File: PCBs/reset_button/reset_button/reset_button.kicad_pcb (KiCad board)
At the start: 2 copper layers, 20 x 40 mm, 3 parts, among them J1 Conn_01x05, SW1 SW_DIP_x02, SW2 SW_DIP_x02

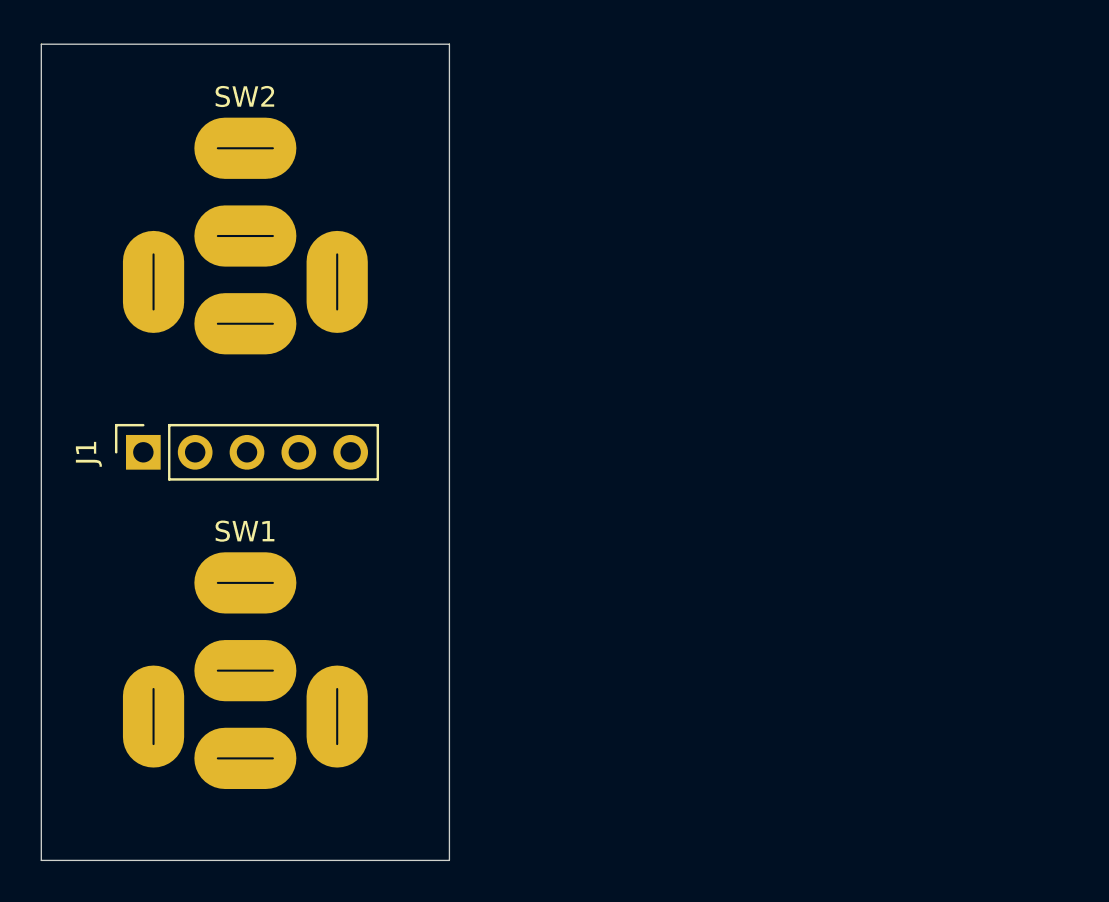
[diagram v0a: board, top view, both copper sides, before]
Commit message: update
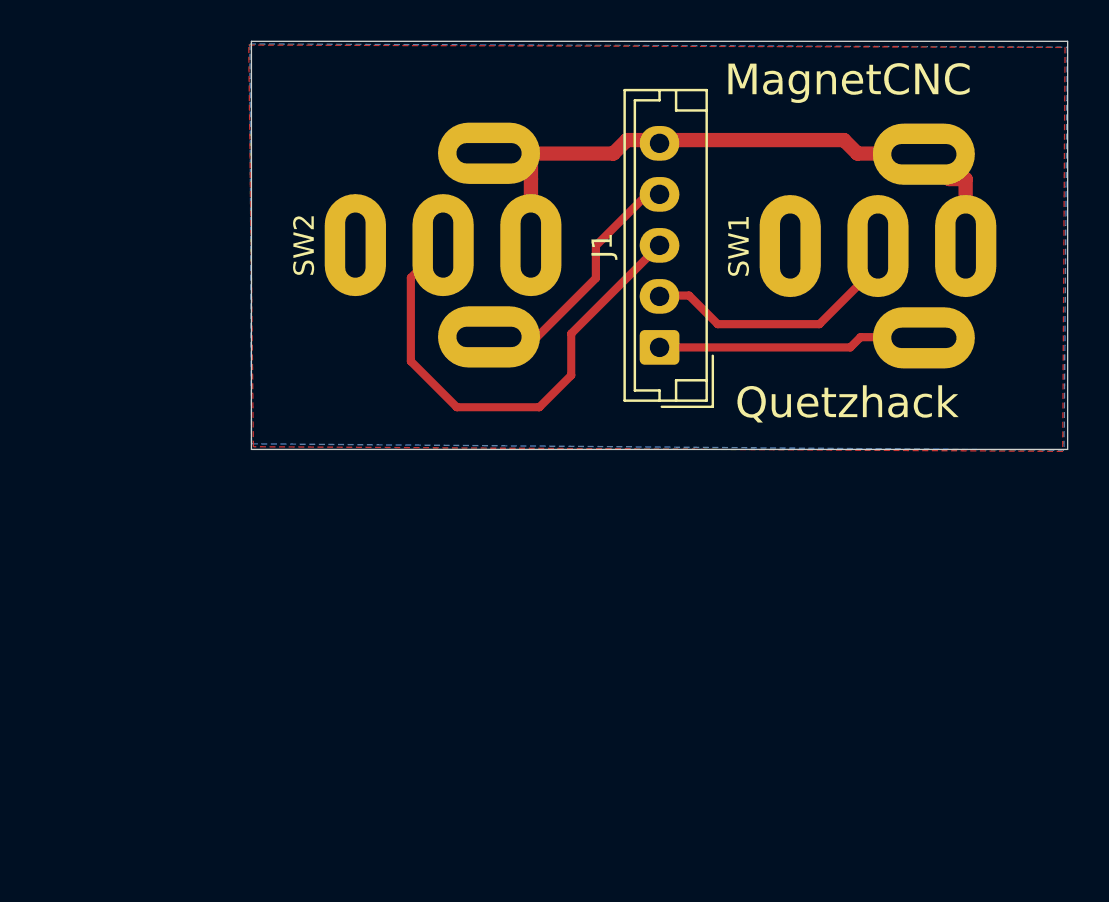
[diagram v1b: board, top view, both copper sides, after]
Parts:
- J1: footprint Connector_PinSocket_2.54mm:PinSocket_1x05_P2.54mm_Vertical -> Connector_JST:JST_EH_B5B-EH-A_1x05_P2.50mm_Vertical
- moved SW1 27.3 mm to (154.7, 92.8), turned to 90 degrees
- moved J1 25.8 mm to (151.3, 97.8)
- moved SW2 8.11 mm to (133.4, 92.7), turned to 90 degrees
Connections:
- J1 pad 3: O_led -> O_sig
- J1 pad 4: O_sig -> O_led
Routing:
- net GND: track 0.00 -> 32.2 mm
- net O_sig: track 0.00 -> 25.7 mm
- net B_sig: track 0.00 -> 13.5 mm
- net B_led: track 0.00 -> 13.2 mm
- net O_led: track 0.00 -> 12.5 mm
- added copper zone on B.Cu, net GND
- added copper zone on F.Cu, net GND
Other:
- board size 20 x 40 mm -> 40 x 20 mm
- net class Default: clearance 0.2 -> 0.4; trace_width 0.25 -> 0.4
- net class gnd added: clearance 0.4, trace_width 0.7, via_dia 0.8, via_drill 0.4
- rule trace_clearance: 0.2 -> 0.4
- board text added: "MagnetCNC"
- board text added: "Quetzhack"
